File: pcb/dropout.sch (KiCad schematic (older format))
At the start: 61 parts, among them SW1 Rotary_Encoder_Switch, SW2 SW_Push, U1 ProMicro

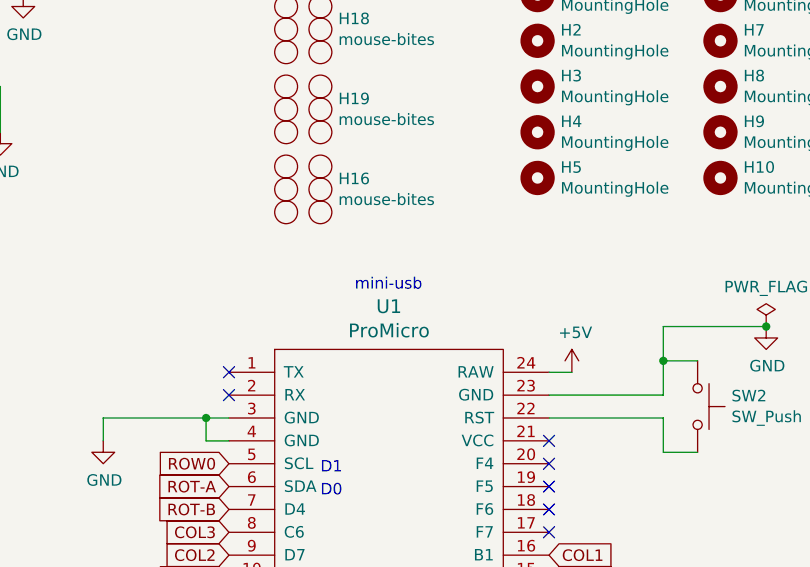
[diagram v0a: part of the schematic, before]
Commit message: adding graphics to pcb, some cleanup
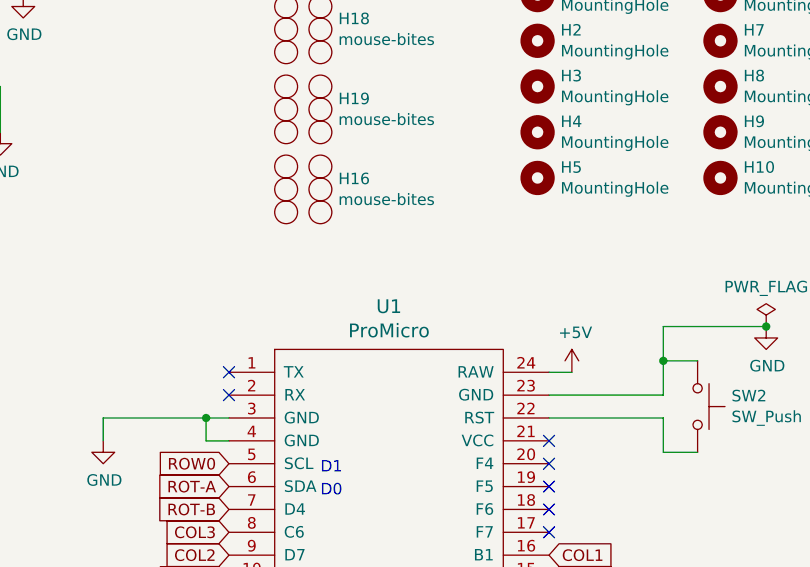
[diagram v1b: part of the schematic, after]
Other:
- note removed: "mini-usb\n"
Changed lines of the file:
@@
 Text Notes 9950 1200 0    50   ~ 0
 Holes for Base
-Text Notes 7700 2650 0    50   ~ 0
-mini-usb\n
 $Comp
 L MX_Alps_Hybrid:MX-NoLED K-FN1
